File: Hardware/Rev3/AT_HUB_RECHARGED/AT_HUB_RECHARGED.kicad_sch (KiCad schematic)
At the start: 31 parts, among them SW1 SW_Push, SW10 SW_Push, SW2 SW_Push, SW3 SW_Push, SW4 SW_Push, SW5 SW_Push, SW6 SW_Push, SW7 SW_Push, SW8 SW_Push, SW9 SW_Push, U1 ESP32-PICO-DEVKITM-2

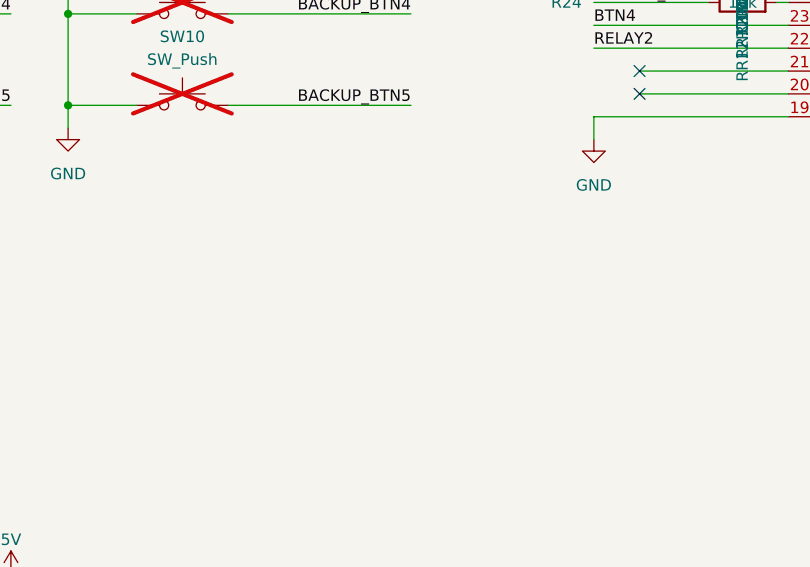
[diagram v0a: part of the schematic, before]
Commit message: Final working
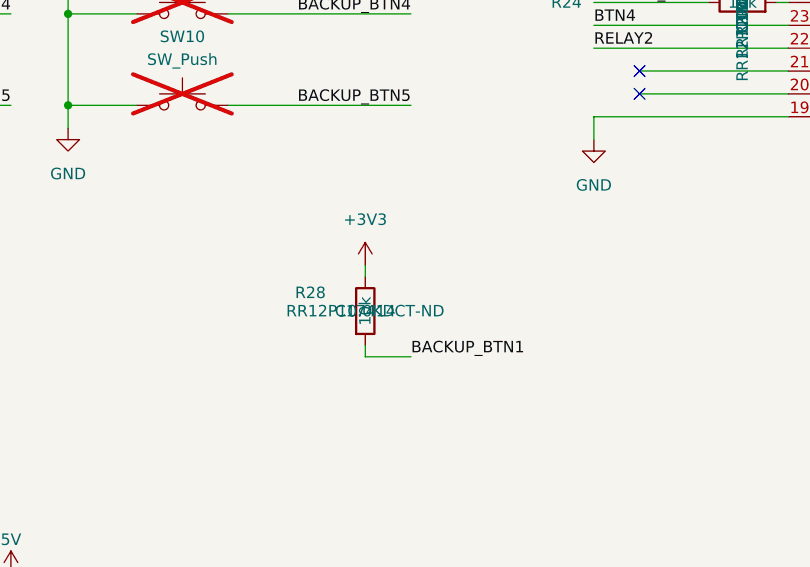
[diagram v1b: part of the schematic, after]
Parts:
- added R28: 10k, Resistor_SMD:R_0805_2012Metric, symbol Device:R
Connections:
- net +3V3: now also R28.1
- net BACKUP_BTN1: now also R28.2
